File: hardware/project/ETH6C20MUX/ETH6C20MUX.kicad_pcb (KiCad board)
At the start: 4 copper layers, 160 x 100 mm, 201 parts, among them J301 5499141-4, J501 Conn_02x06_Odd_Even, J502 Conn_02x08_Odd_Even, J503 C64AC, J601 Conn_02x05, J602 Conn_02x01, K301 HE3621A0510, K302 HE3621A0510, K303 HE3621A0510, K304 HE3621A0510, K305 HE3621A0510, K306 HE3621A0510, K307 HE3621A0510, K308 HE3621A0510, K309 HE3621A0510, K310 HE3621A0510, K311 HE3621A0510, K312 HE3621A0510, K313 HE3621A0510, K314 HE3621A0510, K315 HE3621A0510, K316 HE3621A0510, K317 HE3621A0510, K318 HE3621A0510, K319 HE3621A0510, K320 HE3621A0510, K321 HE3621A0510, K322 HE3621A0510, K323 HE3621A0510, K324 HE3621A0510, K325 HE3621A0510, K326 HE3621A0510, K327 HE3621A0510, K328 HE3621A0510, K329 HE3621A0510, K330 HE3621A0510, K331 HE3621A0510, K332 HE3621A0510, K333 HE3621A0510, K334 HE3621A0510, K335 HE3621A0510, K336 HE3621A0510, K337 HE3621A0510, K338 HE3621A0510, K339 HE3621A0510, K340 HE3621A0510, K341 HE3621A0510, K342 HE3621A0510, K343 HE3621A0510, K344 HE3621A0510, K345 HE3621A0510, K346 HE3621A0510, K347 HE3621A0510, K348 HE3621A0510, K349 HE3621A0510, K350 HE3621A0510, K351 HE3621A0510, K352 HE3621A0510, K353 HE3621A0510, K354 HE3621A0510, K355 HE3621A0510, K356 HE3621A0510, K357 HE3621A0510, K358 HE3621A0510, K359 HE3621A0510, K360 HE3621A0510, K361 HE3621A0510, K362 HE3621A0510, K363 HE3621A0510, K364 HE3621A0510, K365 HE3621A0510, K366 HE3621A0510, K367 HE3621A0510, K368 HE3621A0510, K369 HE3621A0510, K370 HE3621A0510, Q401 IRFR5410, SW601 A6SN-5104, U201 LC03-3.3, U202 LAN8742A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

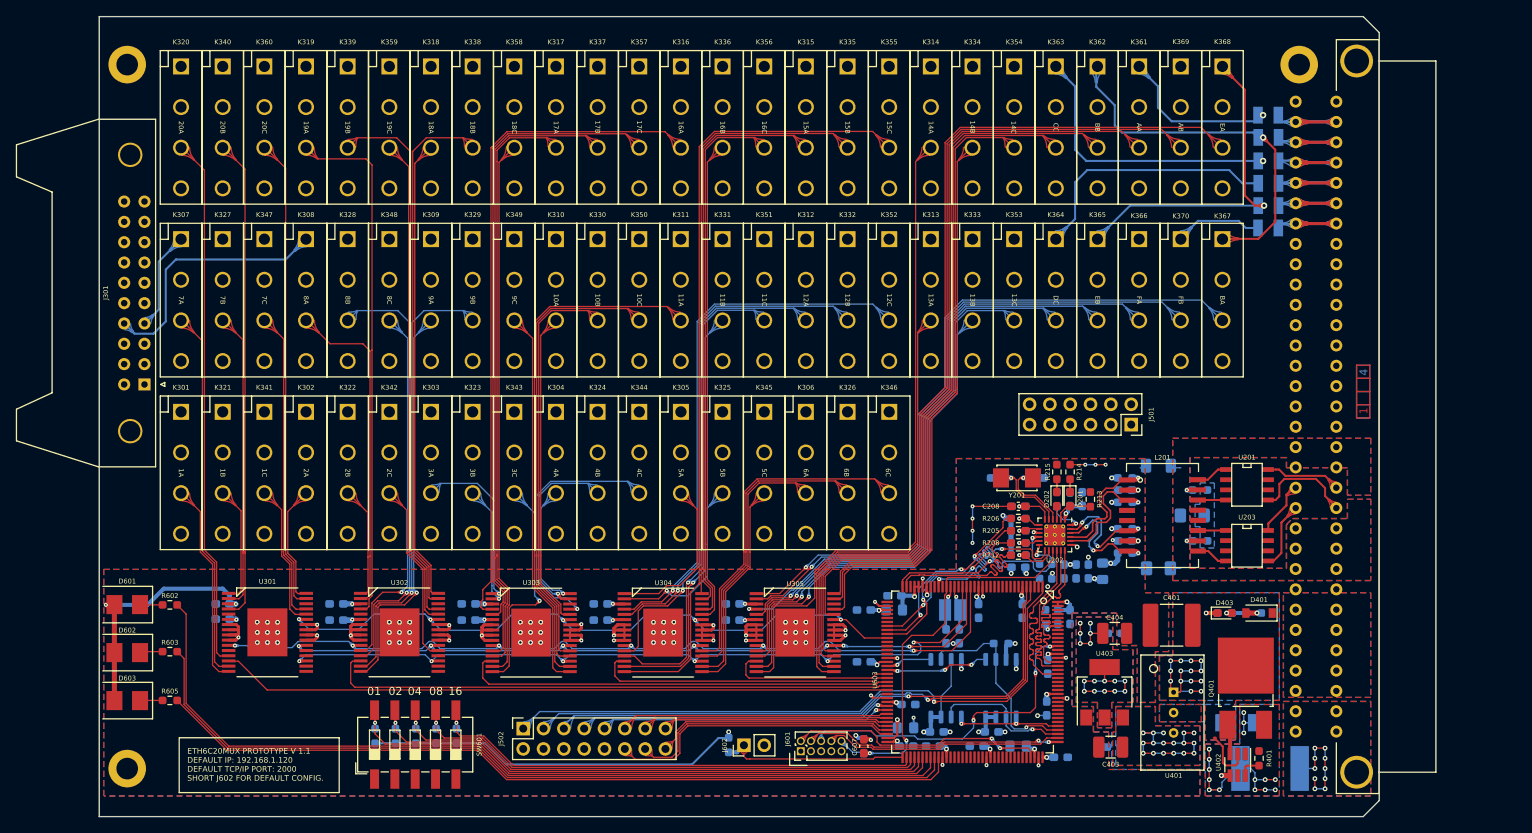
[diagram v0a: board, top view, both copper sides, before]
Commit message: PCB layouts done.
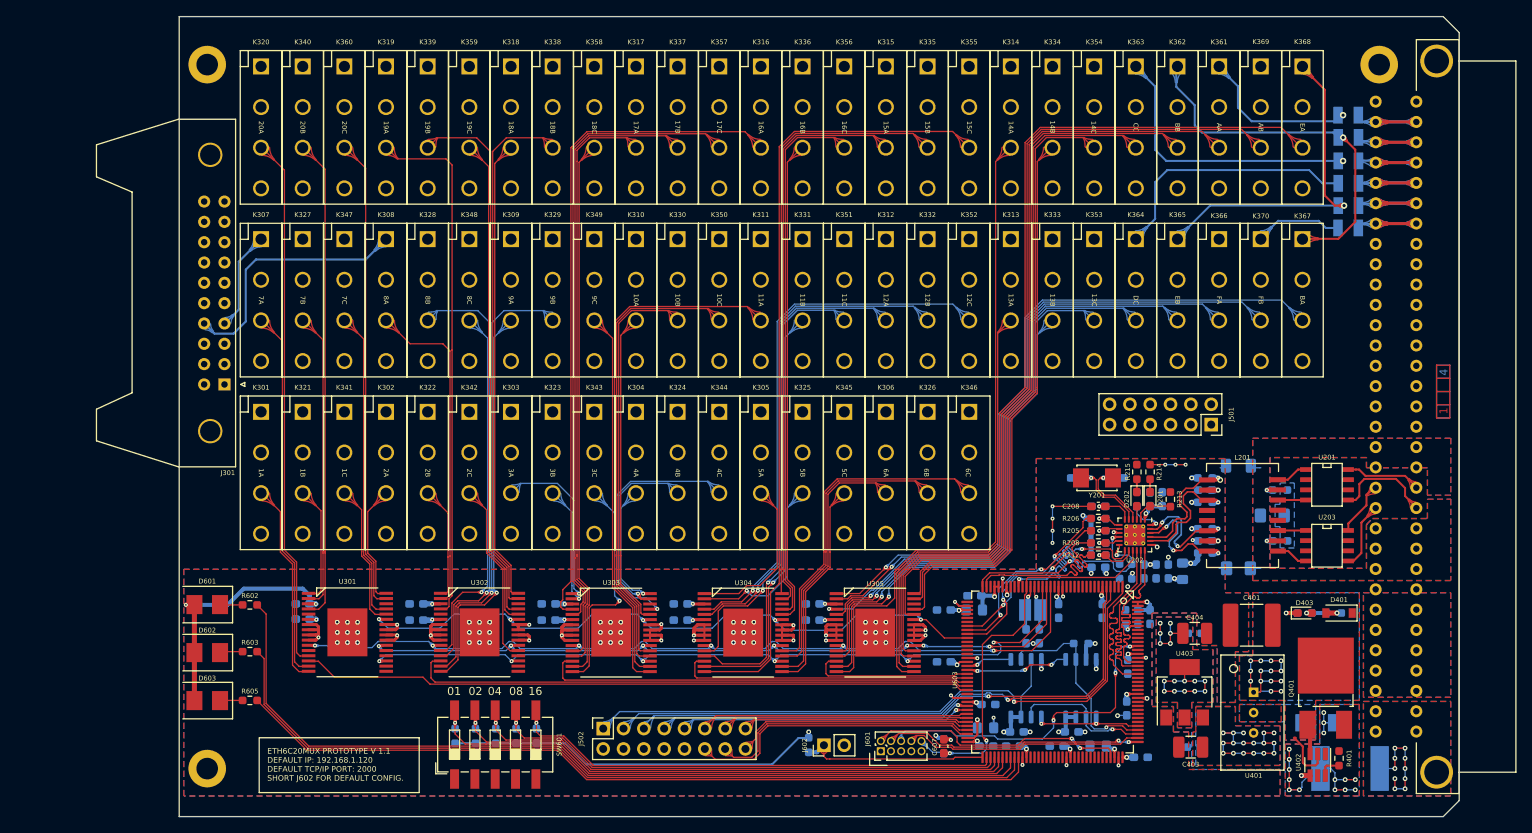
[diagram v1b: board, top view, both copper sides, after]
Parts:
- moved K324 10.0 mm to (132.3, 97.0)
- moved K330 10.0 mm to (132.3, 75.4)
- moved K344 10.0 mm to (137.5, 97.0)
- moved K350 10.0 mm to (137.5, 75.4)
- moved K357 10.0 mm to (137.5, 53.8)
- moved C201 10.0 mm to (193.6, 109.4)
- moved C202 10.0 mm to (184.9, 108.8)
- moved C203 10.0 mm to (191.4, 100.3)
- moved C204 10.0 mm to (192.1, 109.4)
- moved C205 10.0 mm to (192.9, 100.3)
- moved C206 10.0 mm to (190.6, 109.4)
- moved C207 10.0 mm to (198.2, 105.5)
- moved C208 10.0 mm to (184.9, 101.2)
- moved C209 10.0 mm to (184.9, 101.2)
- moved C210 10.0 mm to (198.2, 99.2)
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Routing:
- net /MCU/RELAY1_~CS1: track 71.2 -> 70.6 mm
- net /MCU/RELAY1_~RST: track 86.3 -> 85.8 mm
